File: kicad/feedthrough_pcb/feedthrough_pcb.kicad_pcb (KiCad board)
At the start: 2 copper layers, 150 x 150 mm, 2 parts, among them U1 LSHM-110-02.5-L-DV-A-S-TR, U2 LSHM-110-02.5-L-DV-A-S-TR

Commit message: updated feedthrough pcb
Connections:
- U2 pad 1: Net-(U1-Pad1) -> Net-(U2-Pad1)
- U2 pad 11: Net-(U1-Pad11) -> Net-(U2-Pad11)
- U2 pad 13: Net-(U1-Pad13) -> Net-(U2-Pad13)
- U2 pad 15: Net-(U1-Pad15) -> Net-(U2-Pad15)
- U2 pad 17: Net-(U1-Pad17) -> Net-(U2-Pad17)
- U2 pad 19: Net-(U1-Pad19) -> Net-(U2-Pad19)
- U2 pad 3: Net-(U1-Pad3) -> Net-(U2-Pad3)
- U2 pad 5: Net-(U1-Pad5) -> Net-(U2-Pad5)
- U2 pad 7: Net-(U1-Pad7) -> Net-(U2-Pad7)
- U2 pad 9: Net-(U1-Pad9) -> Net-(U2-Pad9)
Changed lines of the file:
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@@
     (zones 0)
     (modules 2)
-    (nets 21)
+    (nets 31)
   )
   (page A4)
@@
   )
   (setup
-    (last_trace_width 0.1524)
+    (last_trace_width 0.25)
     (user_trace_width 0.1524)
     (trace_clearance 0.2)
@@
     (solder_mask_min_width 0.25)
     (aux_axis_origin 0 0)
-    (visible_elements FFFFFF7F)
+    (visible_elements 7FFFFFFF)
     (pcbplotparams
       (layerselection 0x010fc_ffffffff)
@@
   (net 19 "Net-(U1-Pad19)")
   (net 20 "Net-(U1-Pad20)")
+  (net 21 "Net-(U2-Pad19)")
+  (net 22 "Net-(U2-Pad17)")
+  (net 23 "Net-(U2-Pad15)")
+  (net 24 "Net-(U2-Pad13)")
+  (net 25 "Net-(U2-Pad11)")
+  (net 26 "Net-(U2-Pad9)")
+  (net 27 "Net-(U2-Pad7)")
+  (net 28 "Net-(U2-Pad5)")
+  (net 29 "Net-(U2-Pad3)")
+  (net 30 "Net-(U2-Pad1)")
   (net_class Default "This is the default net class."
     (clearance 0.2)
@@
     (add_net "Net-(U1-Pad8)")
     (add_net "Net-(U1-Pad9)")
+    (add_net "Net-(U2-Pad1)")
+    (add_net "Net-(U2-Pad11)")
+    (add_net "Net-(U2-Pad13)")
+    (add_net "Net-(U2-Pad15)")
+    (add_net "Net-(U2-Pad17)")
+    (add_net "Net-(U2-Pad19)")
+    (add_net "Net-(U2-Pad3)")
+    (add_net "Net-(U2-Pad5)")
+    (add_net "Net-(U2-Pad7)")
+    (add_net "Net-(U2-Pad9)")
   )
   (module feedthrough_pcb:LSHM-110-02.5-L-DV-A-S-TR (layer B.Cu)
@@
       (effects (font (size 1 1) (thickness 0.15)) (justify mirror))
     )
-    (fp_text value LSHM-110-02.5-L-DV-A-S-TR (at 0 3.81) (layer B.Fab) hide
+    (fp_text value LSHM-110-02.5-L-DV-A-S-TR (at 0.1 -5.2) (layer B.Fab) hide
       (effects (font (size 1 1) (thickness 0.15)) (justify mirror))
     )
@@
       (effects (font (size 1 1) (thickness 0.15)))
     )
-    (fp_text value LSHM-110-02.5-L-DV-A-S-TR (at 0 -3.81) (layer F.Fab) hide
+    (fp_text value LSHM-110-02.5-L-DV-A-S-TR (at 0 5.5) (layer F.Fab) hide
       (effects (font (size 1 1) (thickness 0.15)))
     )
@@
       (net 20 "Net-(U1-Pad20)"))
     (pad 19 smd rect (at -2.29 1.75) (size 0.3 1.5) (layers F.Cu F.Paste F.Mask)
-      (net 19 "Net-(U1-Pad19)"))
+      (net 21 "Net-(U2-Pad19)"))
     (pad 18 smd rect (at -1.79 -1.75) (size 0.3 1.5) (layers F.Cu F.Paste F.Mask)
       (net 18 "Net-(U1-Pad18)"))
     (pad 17 smd rect (at -1.79 1.75) (size 0.3 1.5) (layers F.Cu F.Paste F.Mask)
-      (net 17 "Net-(U1-Pad17)"))
+      (net 22 "Net-(U2-Pad17)"))
     (pad 16 smd rect (at -1.29 -1.75) (size 0.3 1.5) (layers F.Cu F.Paste F.Mask)
       (net 16 "Net-(U1-Pad16)"))
     (pad 15 smd rect (at -1.29 1.75) (size 0.3 1.5) (layers F.Cu F.Paste F.Mask)
-      (net 15 "Net-(U1-Pad15)"))
+      (net 23 "Net-(U2-Pad15)"))
     (pad 14 smd rect (at -0.79 -1.75) (size 0.3 1.5) (layers F.Cu F.Paste F.Mask)
       (net 14 "Net-(U1-Pad14)"))
     (pad 13 smd rect (at -0.79 1.75) (size 0.3 1.5) (layers F.Cu F.Paste F.Mask)
-      (net 13 "Net-(U1-Pad13)"))
+      (net 24 "Net-(U2-Pad13)"))
     (pad 12 smd rect (at -0.29 -1.75) (size 0.3 1.5) (layers F.Cu F.Paste F.Mask)
       (net 12 "Net-(U1-Pad12)"))
     (pad 11 smd rect (at -0.29 1.75) (size 0.3 1.5) (layers F.Cu F.Paste F.Mask)
-      (net 11 "Net-(U1-Pad11)"))
+      (net 25 "Net-(U2-Pad11)"))
     (pad 10 smd rect (at 0.21 -1.75) (size 0.3 1.5) (layers F.Cu F.Paste F.Mask)
       (net 10 "Net-(U1-Pad10)"))
     (pad 9 smd rect (at 0.21 1.75) (size 0.3 1.5) (layers F.Cu F.Paste F.Mask)
-      (net 9 "Net-(U1-Pad9)"))
+      (net 26 "Net-(U2-Pad9)"))
     (pad 8 smd rect (at 0.71 -1.75) (size 0.3 1.5) (layers F.Cu F.Paste F.Mask)
       (net 8 "Net-(U1-Pad8)"))
     (pad 7 smd rect (at 0.71 1.75) (size 0.3 1.5) (layers F.Cu F.Paste F.Mask)
-      (net 7 "Net-(U1-Pad7)"))
+      (net 27 "Net-(U2-Pad7)"))
     (pad 6 smd rect (at 1.21 -1.75) (size 0.3 1.5) (layers F.Cu F.Paste F.Mask)
       (net 6 "Net-(U1-Pad6)"))
     (pad 5 smd rect (at 1.21 1.75) (size 0.3 1.5) (layers F.Cu F.Paste F.Mask)
-      (net 5 "Net-(U1-Pad5)"))
+      (net 28 "Net-(U2-Pad5)"))
     (pad 4 smd rect (at 1.71 -1.75) (size 0.3 1.5) (layers F.Cu F.Paste F.Mask)
       (net 4 "Net-(U1-Pad4)"))
     (pad 3 smd rect (at 1.71 1.75) (size 0.3 1.5) (layers F.Cu F.Paste F.Mask)
-      (net 3 "Net-(U1-Pad3)"))
+      (net 29 "Net-(U2-Pad3)"))
     (pad 2 smd rect (at 2.21 -1.75) (size 0.3 1.5) (layers F.Cu F.Paste F.Mask)
       (net 2 "Net-(U1-Pad2)"))
     (pad 1 smd rect (at 2.21 1.75) (size 0.3 1.5) (layers F.Cu F.Paste F.Mask)
-      (net 1 "Net-(U1-Pad1)"))
+      (net 30 "Net-(U2-Pad1)"))
   )
   (gr_circle (center 99.96 97.25) (end 174.96 97.25) (layer Edge.Cuts) (width 0.05))
-  (via (at 97.71 95) (size 0.5048) (drill 0.3) (layers F.Cu B.Cu) (net 20))
-  (via (at 98.21 99.5) (size 0.5048) (drill 0.3) (layers F.Cu B.Cu) (net 18))
-  (via (at 99.21 99.5) (size 0.5048) (drill 0.3) (layers F.Cu B.Cu) (net 14))
-  (via (at 100.21 99.5) (size 0.5048) (drill 0.3) (layers F.Cu B.Cu) (net 10))
-  (via (at 101.21 99.5) (size 0.5048) (drill 0.3) (layers F.Cu B.Cu) (net 6))
   (via (at 102.21 99.5) (size 0.5048) (drill 0.3) (layers F.Cu B.Cu) (net 2))
   (segment (start 102.21 98.25) (end 102.21 99.5) (width 0.1524) (layer F.Cu) (net 2))
@@
   (segment (start 101.71 97.51) (end 101.71 95) (width 0.1524) (layer F.Cu) (net 4))
   (segment (start 101.71 98.25) (end 101.71 97.51) (width 0.1524) (layer F.Cu) (net 4))
+  (via (at 101.21 99.5) (size 0.5048) (drill 0.3) (layers F.Cu B.Cu) (net 6))
   (segment (start 101.21 98.25) (end 101.21 99.5) (width 0.1524) (layer F.Cu) (net 6))
   (segment (start 101.21 96.99) (end 101.21 99.5) (width 0.1524) (layer B.Cu) (net 6))
@@
   (via (at 100.71 95) (size 0.5048) (drill 0.3) (layers F.Cu B.Cu) (net 8))
   (segment (start 100.71 98.25) (end 100.71 95) (width 0.1524) (layer F.Cu) (net 8))
+  (via (at 100.21 99.5) (size 0.5048) (drill 0.3) (layers F.Cu B.Cu) (net 10))
   (segment (start 100.21 98.25) (end 100.21 99.5) (width 0.1524) (layer F.Cu) (net 10))
   (segment (start 100.21 96.25) (end 100.21 99.5) (width 0.1524) (layer B.Cu) (net 10))
@@
   (via (at 99.71 95) (size 0.5048) (drill 0.3) (layers F.Cu B.Cu) (net 12))
   (segment (start 99.71 98.25) (end 99.71 95) (width 0.1524) (layer F.Cu) (net 12))
+  (via (at 99.21 99.5) (size 0.5048) (drill 0.3) (layers F.Cu B.Cu) (net 14))
   (segment (start 99.21 98.25) (end 99.21 99.5) (width 0.1524) (layer F.Cu) (net 14))
   (segment (start 99.21 96.25) (end 99.21 99.5) (width 0.1524) (layer B.Cu) (net 14))
@@
   (via (at 98.71 95) (size 0.5048) (drill 0.3) (layers F.Cu B.Cu) (net 16))
   (segment (start 98.71 98.25) (end 98.71 95) (width 0.1524) (layer F.Cu) (net 16))
+  (via (at 98.21 99.5) (size 0.5048) (drill 0.3) (layers F.Cu B.Cu) (net 18))
   (segment (start 98.21 98.25) (end 98.21 99.5) (width 0.1524) (layer F.Cu) (net 18))
   (segment (start 98.21 96.25) (end 98.21 99.5) (width 0.1524) (layer B.Cu) (net 18))
+  (via (at 97.71 95) (size 0.5048) (drill 0.3) (layers F.Cu B.Cu) (net 20))
   (segment (start 97.71 96.25) (end 97.71 95) (width 0.1524) (layer B.Cu) (net 20))
   (segment (start 97.71 97.3476) (end 97.71 95) (width 0.1524) (layer F.Cu) (net 20))

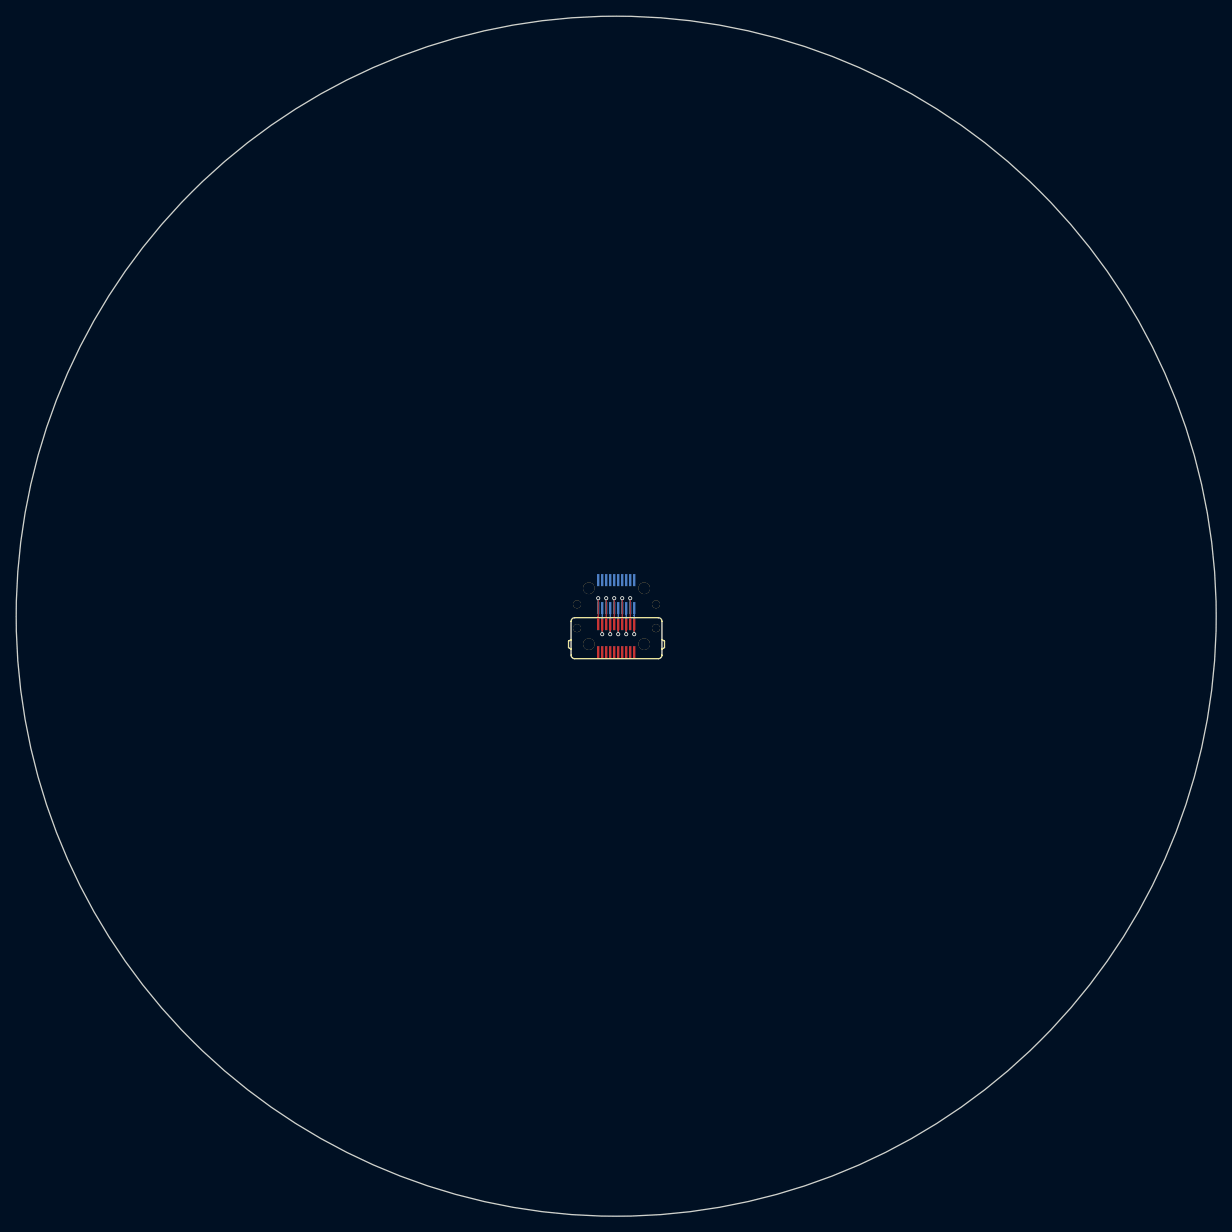
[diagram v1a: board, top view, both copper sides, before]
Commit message: updated feedthrough pcb
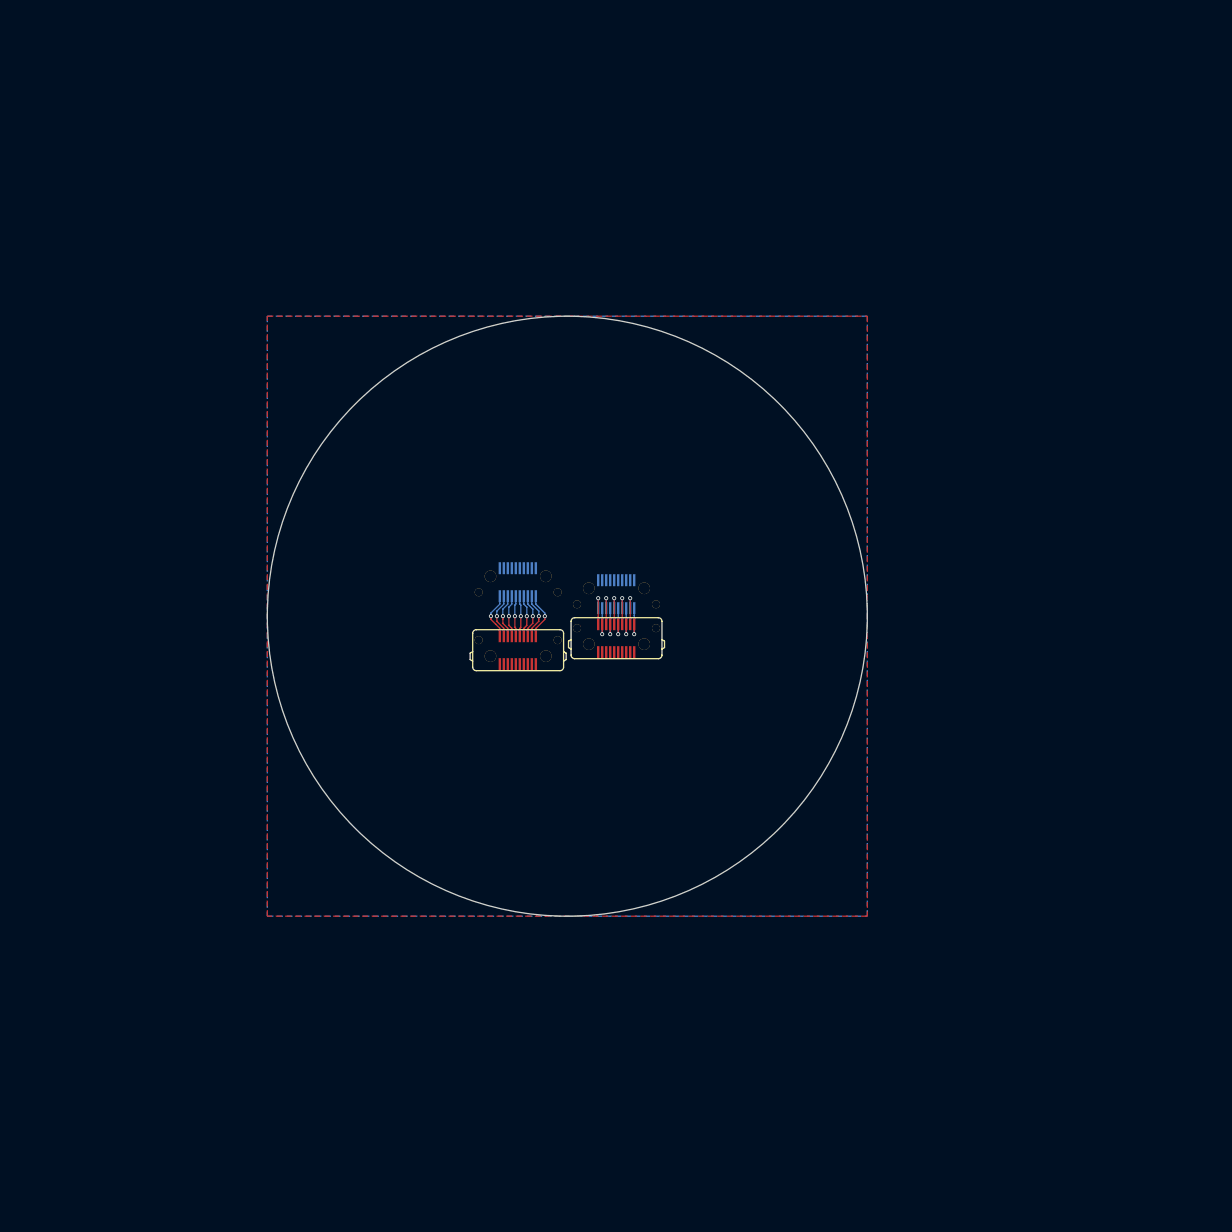
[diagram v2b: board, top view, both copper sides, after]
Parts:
- added U3: LSHM-110-02.5-L-DV-A-S-TR, feedthrough_pcb:LSHM-110-02.5-L-DV-A-S-TR, B.Cu at (87.7, 93.0)
- added U4: LSHM-110-02.5-L-DV-A-S-TR, feedthrough_pcb:LSHM-110-02.5-L-DV-A-S-TR, F.Cu at (87.7, 101.5)
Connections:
- U1 pad 1: Net-(U1-Pad1) -> GND
- U1 pad 11: Net-(U1-Pad11) -> GND
- U1 pad 13: Net-(U1-Pad13) -> GND
- U1 pad 15: Net-(U1-Pad15) -> GND
- U1 pad 17: Net-(U1-Pad17) -> GND
- U1 pad 19: Net-(U1-Pad19) -> GND
- U1 pad 3: Net-(U1-Pad3) -> GND
- U1 pad 41: (no net) -> GND
- U1 pad 5: Net-(U1-Pad5) -> GND
- U1 pad 7: Net-(U1-Pad7) -> GND
- U1 pad 9: Net-(U1-Pad9) -> GND
- U2 pad 1: Net-(U2-Pad1) -> GND
- U2 pad 11: Net-(U2-Pad11) -> GND
- U2 pad 13: Net-(U2-Pad13) -> GND
- U2 pad 15: Net-(U2-Pad15) -> GND
- U2 pad 17: Net-(U2-Pad17) -> GND
- U2 pad 19: Net-(U2-Pad19) -> GND
- U2 pad 3: Net-(U2-Pad3) -> GND
- U2 pad 41: (no net) -> GND
- U2 pad 5: Net-(U2-Pad5) -> GND
- U2 pad 7: Net-(U2-Pad7) -> GND
- U2 pad 9: Net-(U2-Pad9) -> GND
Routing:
- net Net-(U3-Pad2): track 0.00 -> 5.93 mm, vias 0 -> 1
- net Net-(U3-Pad20): track 0.00 -> 5.92 mm, vias 0 -> 1
- net Net-(U3-Pad4): track 0.00 -> 5.72 mm, vias 0 -> 1
- net Net-(U3-Pad18): track 0.00 -> 5.72 mm, vias 0 -> 1
- net Net-(U3-Pad6): track 0.00 -> 5.52 mm, vias 0 -> 1
- net Net-(U3-Pad16): track 0.00 -> 5.51 mm, vias 0 -> 1
- net Net-(U3-Pad8): track 0.00 -> 5.31 mm, vias 0 -> 1
- net Net-(U3-Pad14): track 0.00 -> 5.30 mm, vias 0 -> 1
- net Net-(U3-Pad10): track 0.00 -> 5.10 mm, vias 0 -> 1
- net Net-(U3-Pad12): track 0.00 -> 5.10 mm, vias 0 -> 1
- added copper zone on B.Cu, net GND
- added copper zone on F.Cu, net GND
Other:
- board size 150 x 150 mm -> 75 x 75 mm
